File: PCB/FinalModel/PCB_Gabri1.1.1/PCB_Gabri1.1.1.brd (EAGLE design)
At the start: 33.8 x 21.3 mm, 8 parts, among them U1 VEML6030, U2 TXS0104ED, X1 0446200002

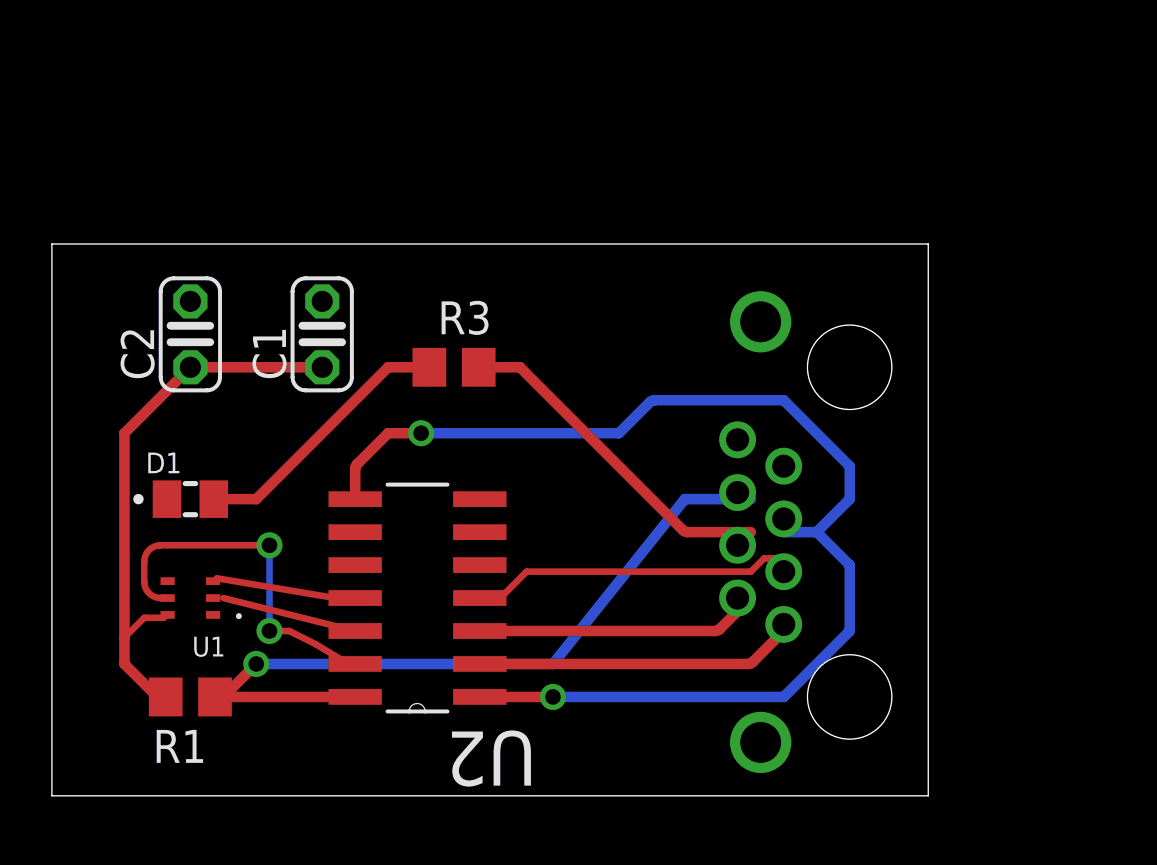
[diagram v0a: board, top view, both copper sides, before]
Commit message: LAB 06022019
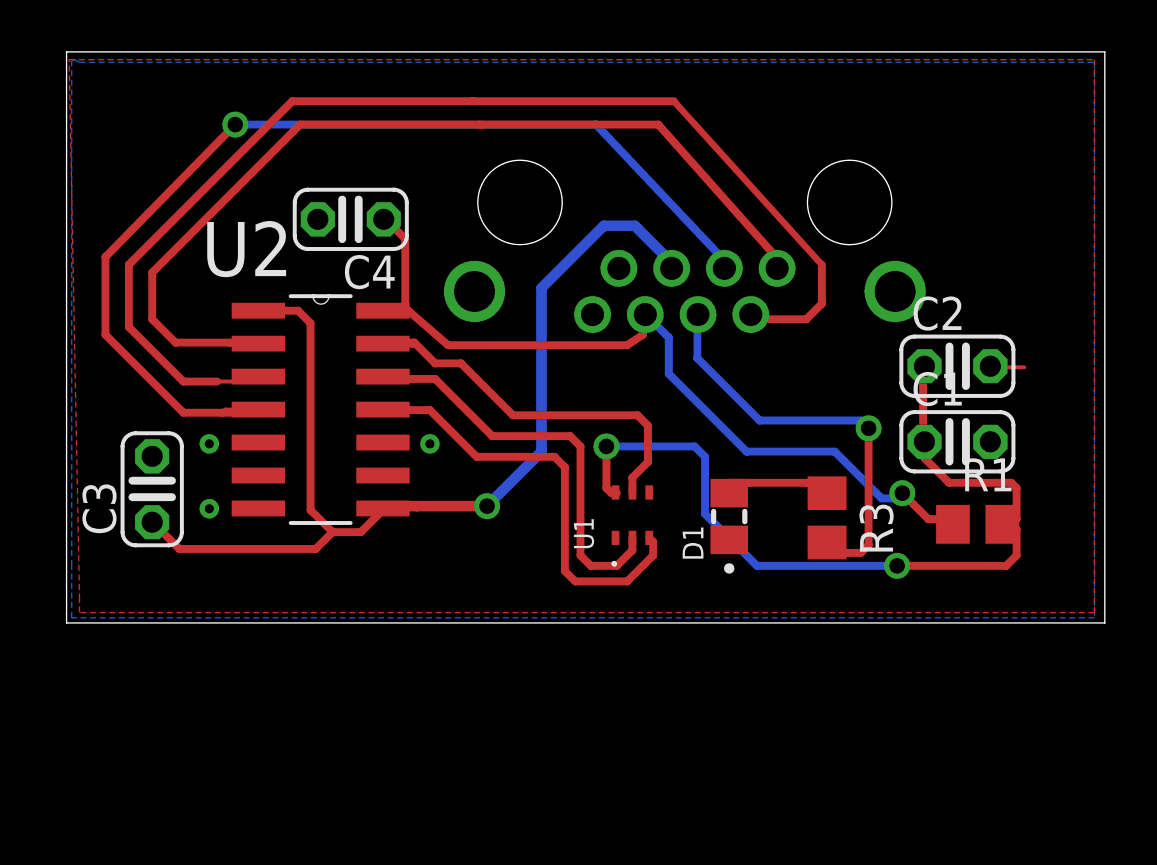
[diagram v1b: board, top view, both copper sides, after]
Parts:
- added C3, C4: (no value), resistor:C025-024X044
- moved R1 31.1 mm to (95.1, 63.8), turned to 0 degrees
- moved C2 29.6 mm to (94.3, 69.9), turned to 0 degrees
- moved C1 24.8 mm to (94.3, 67.0), turned to 0 degrees
- moved D1 20.8 mm to (85.5, 64.1), turned to 90 degrees
- moved U1 17.3 mm to (81.8, 64.2), turned to 90 degrees
- moved R3 15.5 mm to (89.3, 64.0), turned to 270 degrees
- moved X1 14.2 mm to (83.8, 76.2), turned to 180 degrees
- moved U2 1.13 mm to (72.2, 64.4), turned to 0 degrees
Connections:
- net N$1 renamed LS_VDD
- net N$12 renamed LED_1
- net N$3 renamed SCL
- net N$4 renamed INT
- net N$5 renamed SDA
- net N$6 renamed LED_2
- net N$7 renamed A1
- net N$8 renamed A2
- net N$9 renamed A3
- removed net N$10: R1.1, U2.14, X1.6
- removed net N$17: U2.1, U2.8, X1.5
- new net VCCA: C3.1, U2.1, U2.8, X1.5
- new net VCCB: C4.1, R1.1, U2.14, X1.6
- net GND: now also C1.2, C2.2, C3.2, C4.2, D1.C, U1.4, U2.10, U2.5, U2.7, X1.8
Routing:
- net N$17: track 46.1 -> 0.00 mm, vias 2 -> 0
- net A2: track 0.00 -> 45.2 mm
- net VCCA: track 0.00 -> 41.5 mm, vias 0 -> 1
- net A3: track 0.00 -> 39.5 mm, vias 0 -> 1
- net A1: track 0.00 -> 36.2 mm
- net VCCB: track 0.00 -> 32.9 mm, vias 0 -> 1
- net N$10: track 29.0 -> 0.00 mm, vias 1 -> 0
- net INT: track 0.00 -> 16.6 mm
- net LED_1: track 0.00 -> 16.5 mm, vias 0 -> 1
- net SCL: track 0.00 -> 15.0 mm
- net N$18: track 13.6 -> 0.00 mm, vias 2 -> 0
- net N$2: track 12.8 -> 0.00 mm
- net N$15: track 11.9 -> 0.00 mm
- net N$11: track 11.8 -> 0.00 mm
- net LS_VDD: track 21.2 -> 32.0 mm, vias 0 -> 2
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- added copper zone on layer 1, net GND
- added copper zone on layer 16, net GND
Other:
- board size 33.8 x 21.3 mm -> 40 x 22 mm
